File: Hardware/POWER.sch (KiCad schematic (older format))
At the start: 28 parts, among them J1 ATX24, J2 ATX24, P1 RCA_Stero_Jack, P2 RCA_Stero_Jack, P3 3.5mm_Audio, P4 3.5mm_Audio, Q2 BSS138, SW1 PWR_BTN, U2 LP38692, U3 PLR135/T10, U4 POM-3535L-3-R, U5 POM-3535L-3-R, U6 PLT133/T10W, U7 POM-3535L-3-R, U8 POM-3535L-3-R

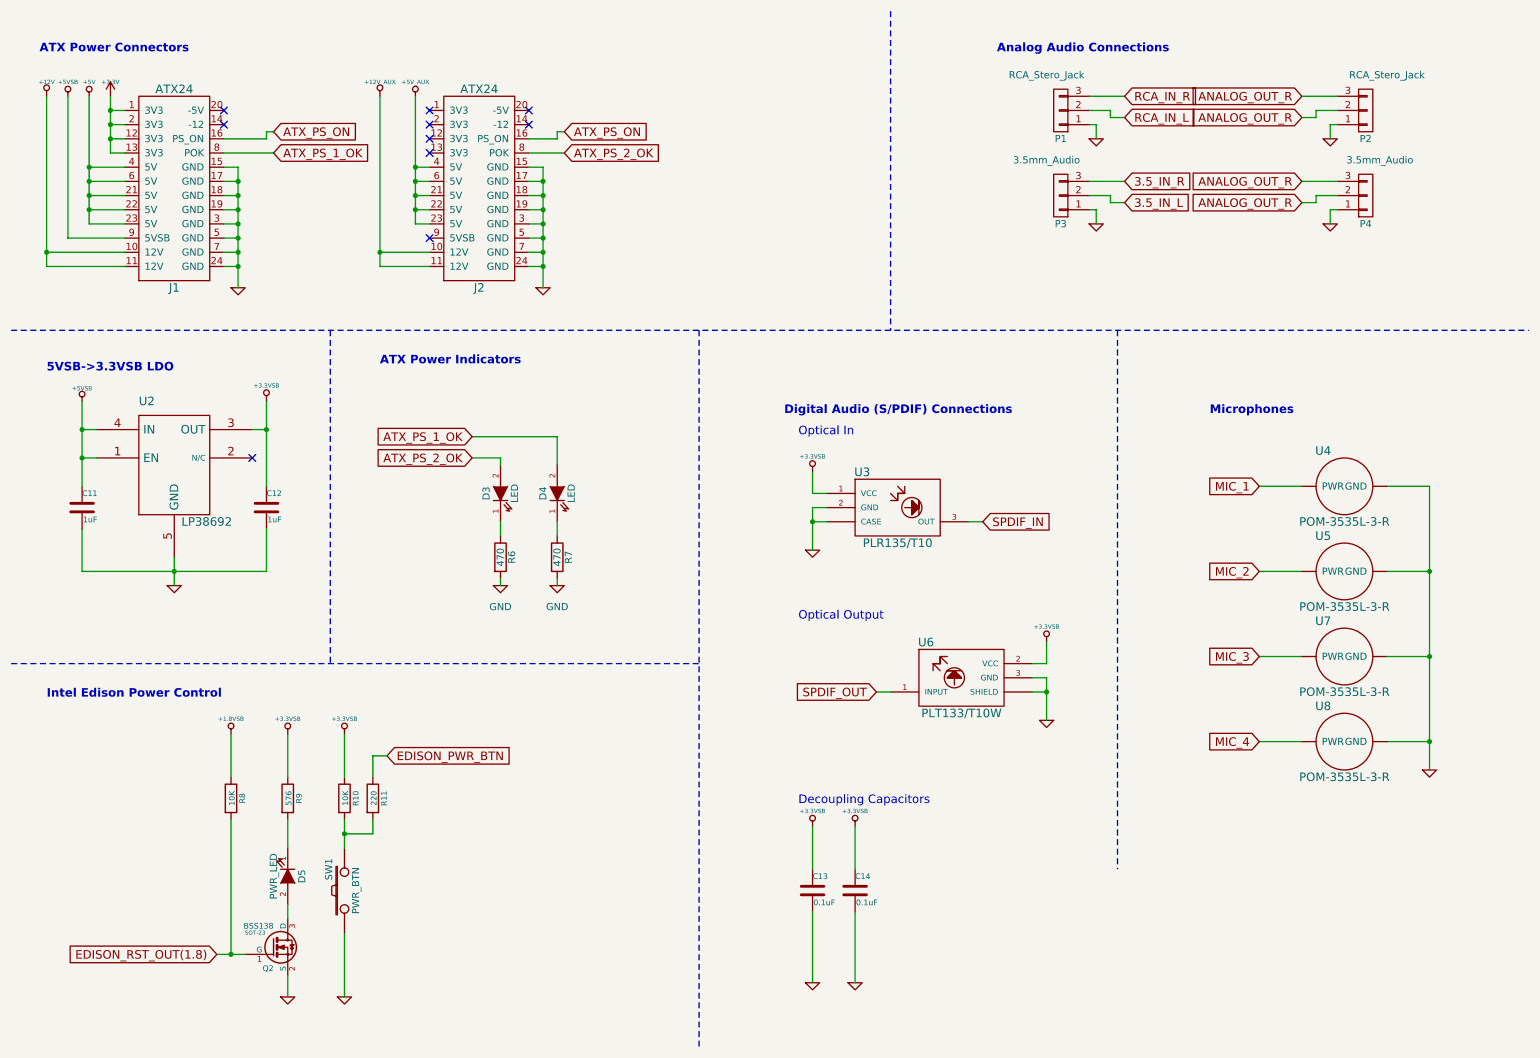
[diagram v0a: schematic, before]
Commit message: Pushing most updated version
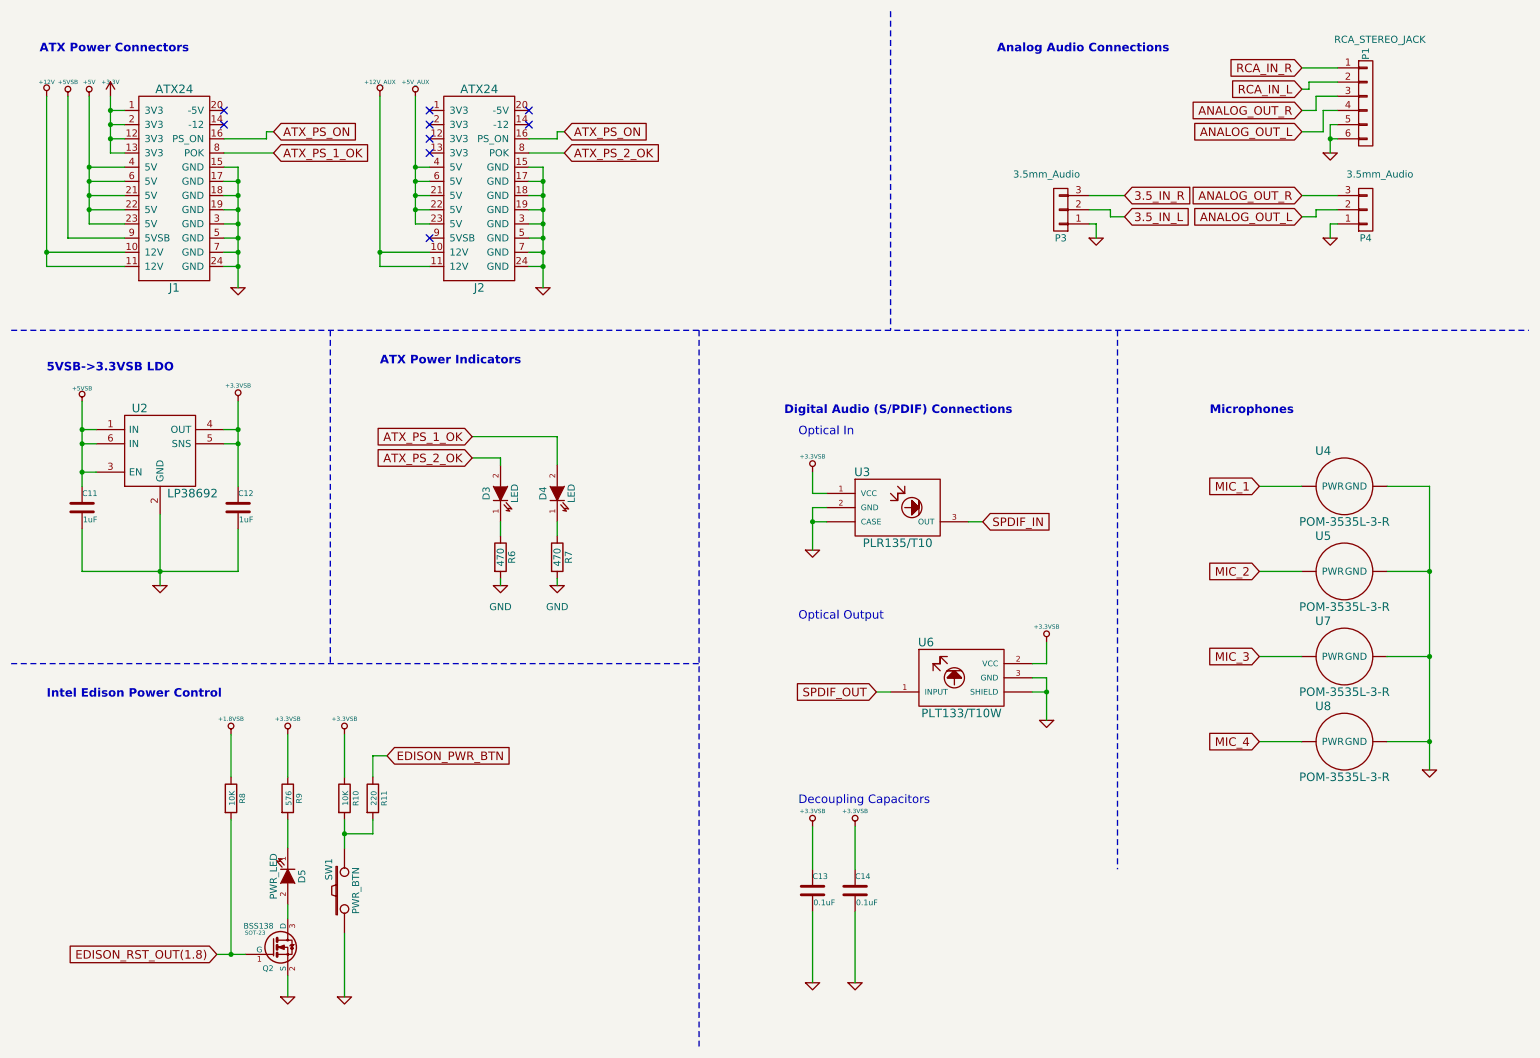
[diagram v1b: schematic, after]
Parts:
- removed P1, P2: RCA_Stero_Jack, symbol RCA_Stero_Jack
- removed U2: LP38692, symbol LP38692-RESCUE-museV2
- added P1: RCA_STEREO_JACK, symbol CONN_01X06
- added U2: LP38692, symbol LP38692SD
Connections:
- net +3.3VSB: now also U2.4 (OUT), U2.5 (SNS)
- net +5VSB: now also U2.1 (IN), U2.3 (EN), U2.6 (IN)
- net ANALOG_OUT_R: now also P1.3 (P3); no longer P4.2 (P2)
- net GND: now also P1.5 (P5), P1.6 (P6), U2.2 (GND)
- net RCA_IN_L: now also P1.2 (P2)
- net RCA_IN_R: now also P1.1 (P1)
- new net ANALOG_OUT_L: P1.4 (P4), P4.2 (P2)
- no-connect marks 10 -> 9
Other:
- moved on the sheet: C12, P3, P4
